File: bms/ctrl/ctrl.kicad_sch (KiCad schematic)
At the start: 1 part

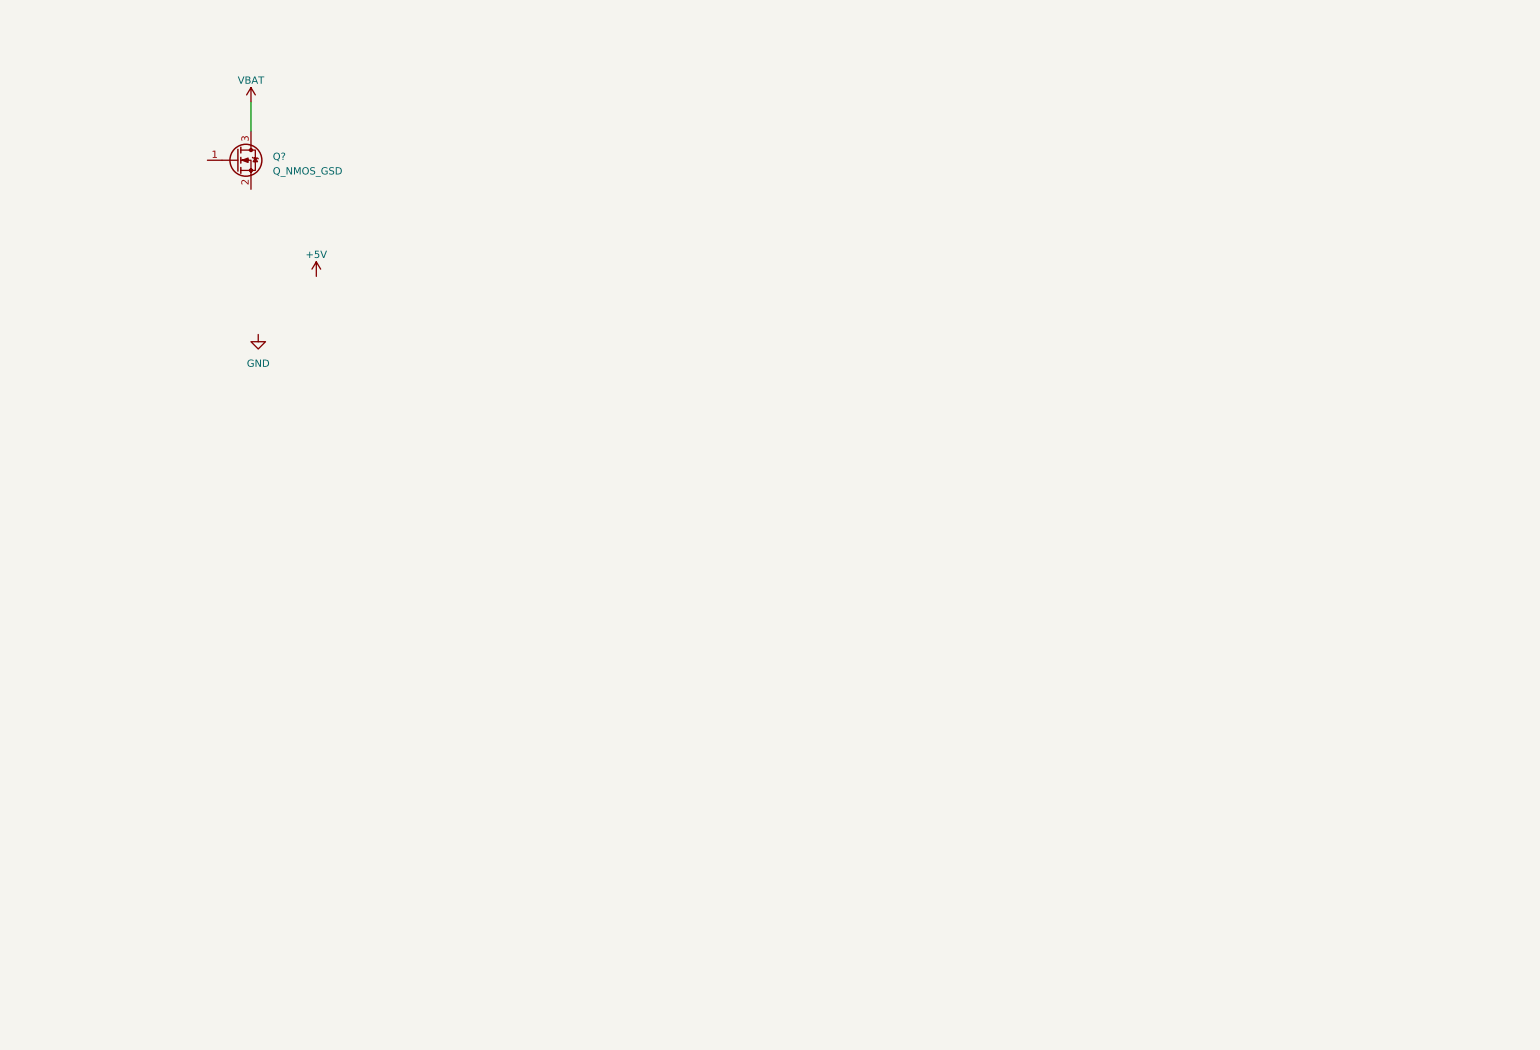
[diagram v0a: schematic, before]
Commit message: BMS stuff update
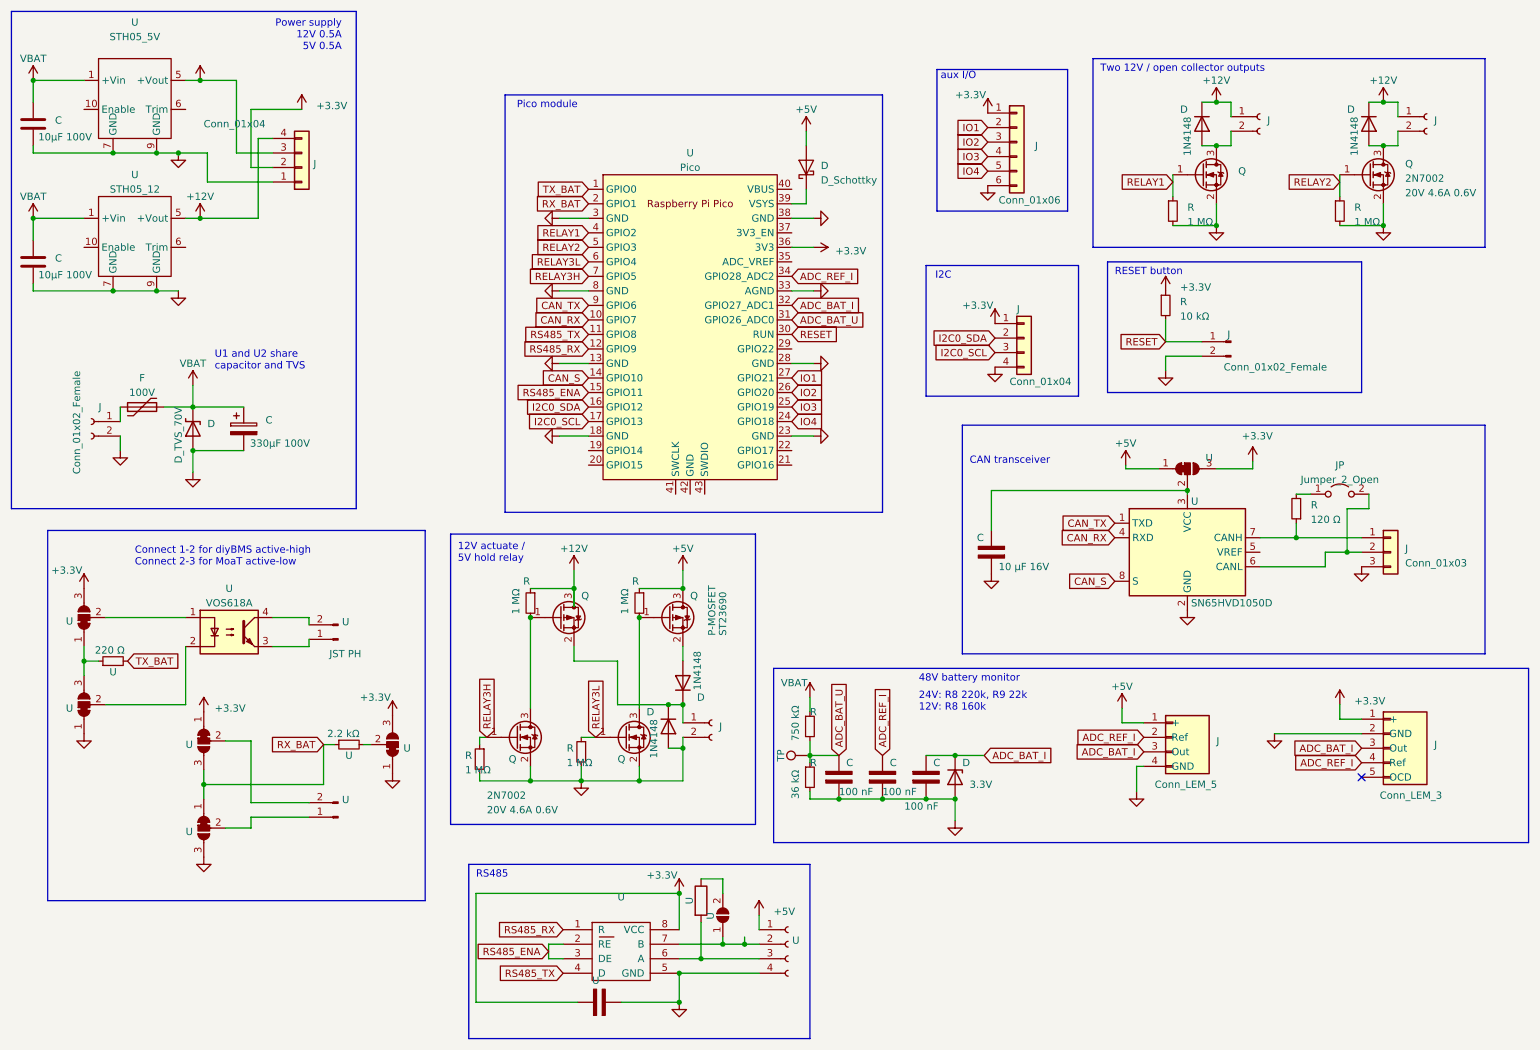
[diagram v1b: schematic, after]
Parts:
- removed Q?: Q_NMOS_GSD, symbol Device:Q_NMOS_GSD
- added C (x2): CP_1µ_100V_0805, Resistor_SMD:R_0805_2012Metric, symbol localparts:CP_10µ_100V_1210
- added C (x3): CP_100n_50V_0603, Capacitor_SMD:C_0603_1608Metric, symbol localparts:CP_100n_50V_0603
- added C: CP_330µ_100V_1210, localstuff:CP_Elec_19x19, symbol localparts:CP_330µ_100V_1210
- added C: CP_10µ_16V_0603, Capacitor_SMD:C_0603_1608Metric, symbol localparts:CP_10µ_16V_0603
- added D (x4): 1N4148, Diode_THT:D_DO-35_SOD27_P7.62mm_Horizontal, symbol Diode:1N4148
- added D: D_Zener_3V3, localstuff:SOD80, symbol localparts:D_Zener_3V3
- added D: D_Schottky, symbol localstuff:D_Schottky
- added D: D_TVS_70V, localstuff:SOD-123FL, symbol localparts:D_TVS_70V
- added F: Polyfuse 100V, Diode_SMD:D_SMA, symbol localparts:Polyfuse 100V
- added J: Conn_01x06, symbol Connector_Generic:Conn_01x06
- added J (x4): Conn_01x02_Female, symbol Connector:Conn_01x02_Female
- added J (x2): Conn_01x04, symbol Connector_Generic:Conn_01x04
- added J: Conn_LEM_5, Connector_JST:JST_PH_B4B-PH-K_1x04_P2.00mm_Vertical, symbol localstuff:Conn_LEM_5
- added J: Conn_01x02_Female, symbol Connector:Conn_01x02_Male
- added J: Conn_LEM_3, Connector_JST:JST_PH_B5B-PH-K_1x05_P2.00mm_Vertical, symbol localstuff:Conn_LEM_3
- added J: Conn_01x03, symbol Connector_Generic:Conn_01x03
- added JP: Jumper_2_Open, symbol Jumper:Jumper_2_Open
- added Q (x2): ST23690, Package_DFN_QFN:AO_DFN-8-1EP_5.55x5.2mm_P1.27mm_EP4.12x4.6mm, symbol Transistor_FET:BSS83P
- added Q (x4): 2N7002, Package_TO_SOT_SMD:SOT-23, symbol localparts:Q_NMOS_20V_4A_lowVth
- added R: R_120_0603, Resistor_SMD:R_0603_1608Metric, symbol localparts:R_120_0603
- added R: R_10k_0603, Resistor_SMD:R_0603_1608Metric, symbol localparts:R_10k_0603
- added R (x6): R_1M_0603, Resistor_SMD:R_0603_1608Metric, symbol localparts:R_1M_0603
- added R: R_36k_0603_1, Resistor_SMD:R_0603_1608Metric, symbol localparts:R_36k_0603_1
- added R: R_750k_0603, Resistor_SMD:R_0603_1608Metric, symbol localparts:R_750k_0603
- added TP: TestPoint, symbol Connector:TestPoint
- added U: SN65HVD1050D, Package_SO:SOIC-8_3.9x4.9mm_P1.27mm, symbol Interface_CAN_LIN:SN65HVD1050D
- added U (x6): (no value), symbol Jumper:SolderJumper_3_Bridged12
- added U: STH05_12, localstuff:STH05, symbol localstuff:STH05_12
- added U: (no value), symbol Jumper:SolderJumper_2_Open
- added U: (no value), symbol ControllerCircuit:SN65HVD75DR
- added U (x2): (no value), symbol Connector:Conn_01x02_Male
- added U: (no value), symbol localparts:R_2k2_0603
- added U: (no value), symbol Device:R
- added U: (no value), symbol Connector:Conn_01x04_Female
- added U: Pico, RPi_Pico:RPi_Pico_SMD_TH, symbol pico:Pico
- added U: (no value), symbol localparts:R_220_0603
- added U: (no value), symbol localparts:CP_100n_50V_0603
- added U: VOS618A, Package_SO:SOP-4_4.4x2.6mm_P1.27mm, symbol localparts:VOS618A
- added U: STH05_5V, localstuff:STH05, symbol localstuff:STH05_5V
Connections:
- net +5V: now also D.2 (A), J.1 (+), J.3 (Pin_3), Q.3 (D), R.1, U.1 (A), U.1 (Pin_1), U.5 (+Vout)
- net GND: now also C.2, C.2, C.2, C.2, C.2, C.2, C.2, D.2 (A), D.2 (A), D.2 (A), J.1 (Pin_1), J.2 (GND), J.2 (Pin_2), J.2 (Pin_2), J.2 (Pin_2), J.3 (Pin_3), J.4 (GND), J.4 (Pin_4), J.6 (Pin_6), Q.2 (S), Q.2 (S), Q.2 (S), Q.2 (S), R.2, R.2, R.2, R.2, R.2, U.1 (A), U.1 (A), U.13 (GND), U.18 (GND), U.2, U.2 (GND), U.23 (GND), U.28 (GND), U.3 (B), U.3 (GND), U.33 (AGND), U.38 (GND), U.4 (Pin_4), U.5 (GND), U.7 (GND), U.7 (GND), U.8 (GND), U.9 (GND), U.9 (GND)
- net VBAT: now also C.1, C.1, C.1, D.1 (K), F.2, R.1, U.1 (+Vin), U.1 (+Vin)
- new net: C.1, U.2 (C), U.3 (VCC)
- new net: J.2 (Pin_2), JP.2 (B), U.6 (CANL)
- new net: J.1 (Pin_1), R.1, U.7 (CANH)
- new net: JP.1 (A), R.2
- new net: F.1, J.1 (Pin_1)
- new net: D.2 (A), J.2 (Pin_2), Q.3 (D) (x2)
- new net: Q.1 (G), Q.3 (D), R.2 (x2)
- new net: D.2 (A), Q.2 (S)
- new net: U.1 (A), U.2 (Pin_2), U.7 (B)
- new net: U.1, U.2 (B)
- new net: U.1, U.1 (A), U.3 (B)
- new net: U.1, U.2 (C)
- new net: D.1 (K), D.1 (K), J.1 (Pin_1), Q.2 (S)
- new net: U.1 (Pin_1), U.2 (C)
- new net: U.2, U.3 (Pin_3), U.6 (A)
- new net: U.1 (Pin_1), U.3
- new net: U.2 (Pin_2), U.4
- new net: U.2, U.2 (C) (x2)
- new net: D.1 (K), U.39 (VSYS)
- new net: U.2 (C), U.2 (Pin_2)
- new net +12V: D.1 (K), D.1 (K), J.1 (Pin_1), J.1 (Pin_1), J.4 (Pin_4), Q.3 (D), R.1, U.5 (+Vout)
- new net +3V3: J.1 (+), J.1 (Pin_1), J.1 (Pin_1), J.2 (Pin_2), R.1, U.1, U.1 (A), U.3 (B), U.3 (B), U.3 (B), U.36 (3V3), U.8 (VCC)
- new net ADC_BAT_I: C.1, D.1 (K), J.3 (Out), J.3 (Out), U.32 (GPIO27_ADC1)
- new net ADC_BAT_U: C.1, R.1, R.2, TP.1, U.31 (GPIO26_ADC0)
- new net ADC_REF_I: C.1, J.2 (Ref), J.4 (Ref), U.34 (GPIO28_ADC2)
- new net CAN_RX: U.10 (GPIO7), U.4 (RXD)
- new net CAN_S: U.14 (GPIO10), U.8 (S)
- new net CAN_TX: U.1 (TXD), U.9 (GPIO6)
- new net I2C0_SCL: J.3 (Pin_3), U.17 (GPIO13)
- new net I2C0_SDA: J.2 (Pin_2), U.16 (GPIO12)
- new net IO1: J.2 (Pin_2), U.27 (GPIO21)
- new net IO2: J.3 (Pin_3), U.26 (GPIO20)
- new net IO3: J.4 (Pin_4), U.25 (GPIO19)
- new net IO4: J.5 (Pin_5), U.24 (GPIO18)
- new net RELAY1: Q.1 (G), R.1, U.4 (GPIO2)
- new net RELAY2: Q.1 (G), R.1, U.5 (GPIO3)
- new net RELAY3H: Q.1 (G), R.1, U.7 (GPIO5)
- new net RELAY3L: Q.1 (G), R.1, U.6 (GPIO4)
- new net RESET: J.1 (Pin_1), R.2, U.30 (RUN)
- new net RS485_ENA: U.15 (GPIO11), U.2 (RE), U.3 (DE)
- new net RS485_RX: U.1 (R), U.12 (GPIO9)
- new net RS485_TX: U.11 (GPIO8), U.4 (D)
- new net RX_BAT: U.1, U.1 (A), U.2 (GPIO1), U.3 (B)
- new net TX_BAT: U.1 (GPIO0), U.2
- no-connect marks 0 -> 1
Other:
- note added: "12V actuate / 5V hold relay"
- note added: "24V: R8 220k, R9 22k 12V: R8 160k"
- note added: "48V battery monitor"
- note added: "CAN transceiver"
- note added: "Connect 1-2 for diyBMS active-high Connect 2-3 for MoaT active-low"
- note added: "I2C"
- note added: "Pico module"
- note added: "Power supply 12V 0.5A 5V 0.5A"
- note added: "RESET button"
- note added: "RS485"
- note added: "Two 12V / open collector outputs"
- note added: "U1 and U2 share capacitor and TVS"
- note added: "aux I/O"

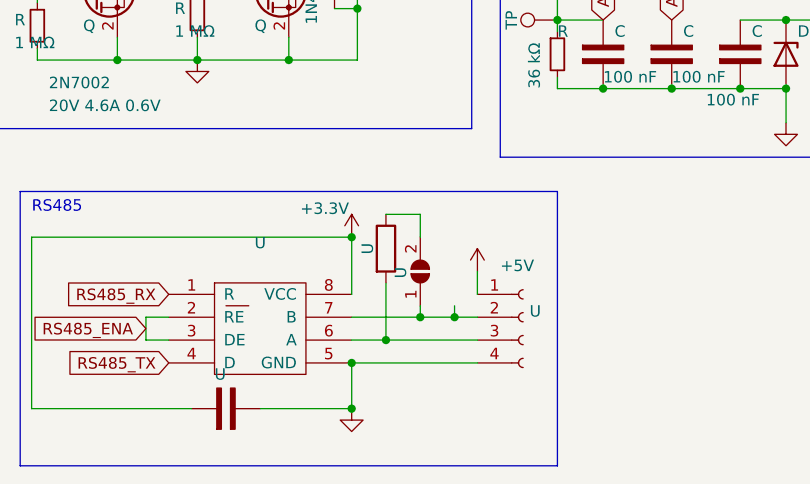
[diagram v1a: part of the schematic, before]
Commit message: minor fixup
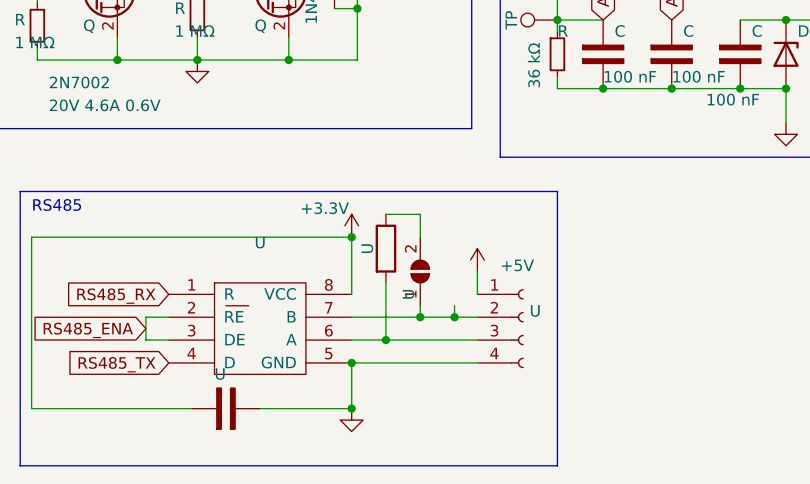
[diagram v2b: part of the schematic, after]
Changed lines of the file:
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@@
     (in_bom yes) (on_board yes)
     (default_instance (reference "U") (unit 1) (value "") (footprint ""))
-    (property "Reference" "U" (id 0) (at 135.001 171.577 0)
+    (property "Reference" "U" (id 0) (at 135.89 173.99 0)
       (effects (font (size 1.27 1.27)))
     )
